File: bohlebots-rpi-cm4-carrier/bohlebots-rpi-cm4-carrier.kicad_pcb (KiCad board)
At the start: 2 copper layers, 32 parts, among them J1 SI-46001-F, J2 power_reference, J3 IO_Conn_02x05, J4 I2C_Conn_1x04, J5 pwr_connector, J6 pwr_connector, K1 Kicker, T1 Taster_LED, T2 Taster_LED, U1 Compute_Module_4_Connectors, U2 USB_Conn_01x05_Pin, U3 DT1446-04SO-7, U5 DT1446-04SO-7, X1 Miromatch

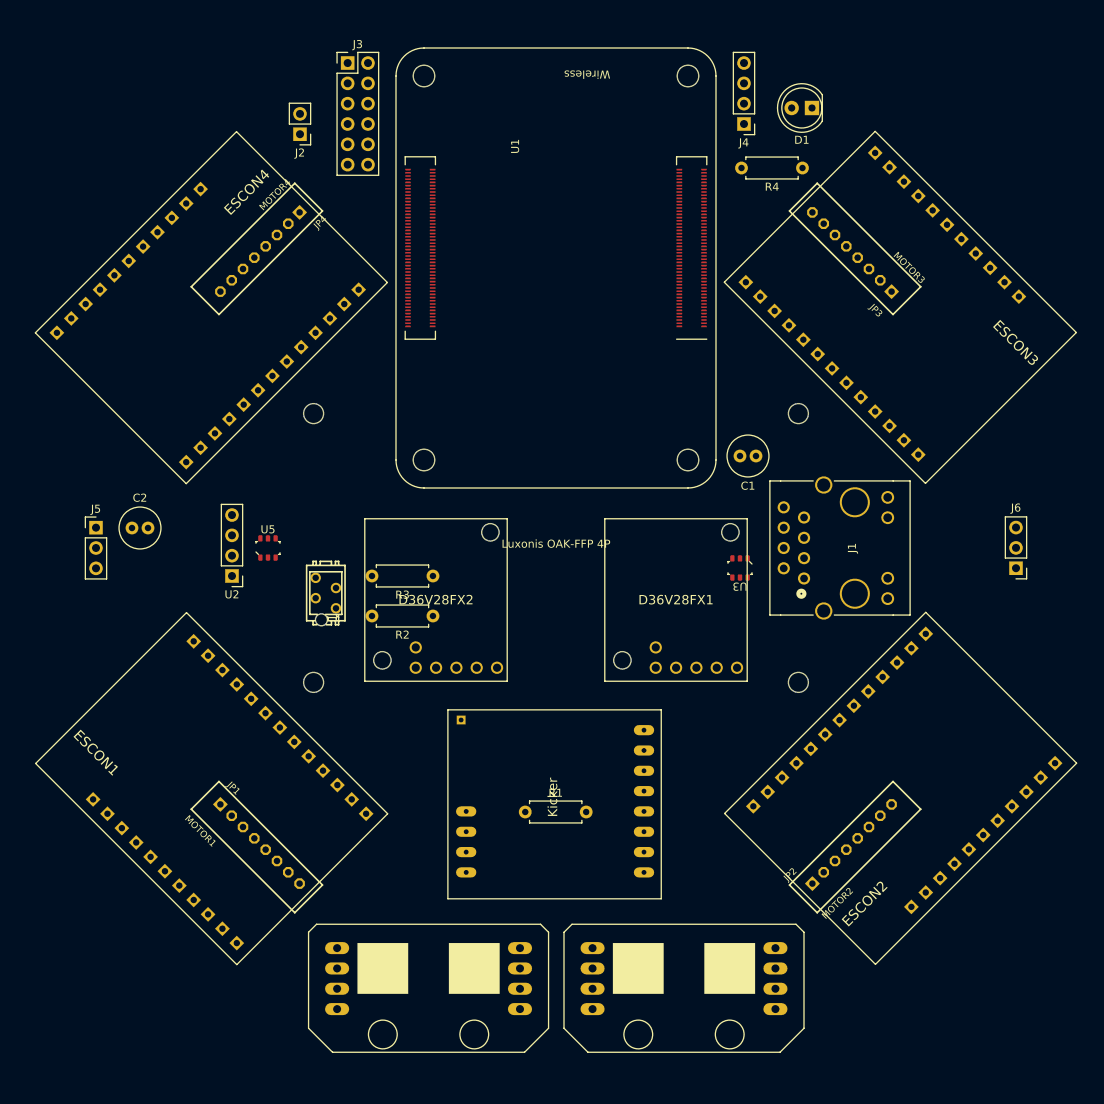
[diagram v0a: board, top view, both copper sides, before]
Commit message: V01 finished.
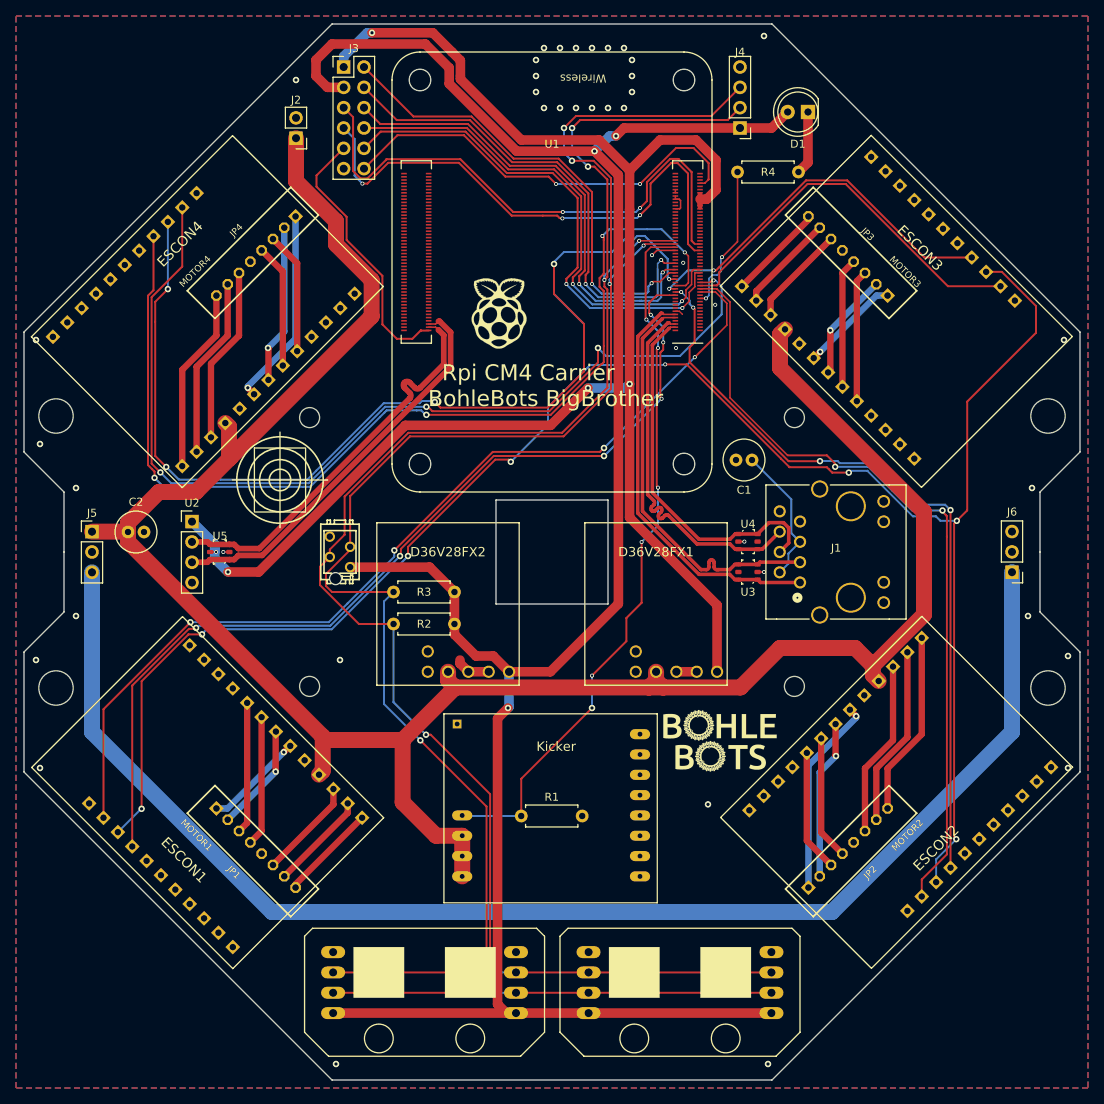
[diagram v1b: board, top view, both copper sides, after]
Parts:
- added G***: LOGO, bohlebots:logo_klein, F.Cu at (126.4, 129.1)
- added G***: LOGO, RPi_Compute_Module_4:logo, F.Cu at (98.9, 75.7)
- added REF**: MountingHole_4.3mm_M4, MountingHole:MountingHole_4.3mm_M4, F.Cu at (167.5, 88.5)
- added REF**: BohlebotsBigBrother_Logo, bohlebots-rpi-cm4-carrier:BohlebotsBigBrother_Logo, F.Cu at (71.5, 96.5)
- added REF**: MountingHole_4.3mm_M4, MountingHole:MountingHole_4.3mm_M4, F.Cu at (43.5, 122.5)
- added REF**: MountingHole_4.3mm_M4, MountingHole:MountingHole_4.3mm_M4, F.Cu at (43.5, 88.5)
- added REFe: MountingHole_4.3mm_M4, MountingHole:MountingHole_4.3mm_M4, F.Cu at (167.5, 122.5)
- added U4: DT1446-04SO-7, bohlebots-rpi-cm4-carrier:SOT26, F.Cu at (130.0, 104.2)
- moved U2 8.44 mm to (60.5, 101.7), turned to 0 degrees
- moved U5 6.05 mm to (64.0, 105.5), turned to 90 degrees
- moved X1 5.44 mm to (77.7, 104.9)
- moved R3 3.35 mm to (93.3, 110.5)
- moved R2 2.87 mm to (93.3, 114.5)
- moved D36V28FX1 2.55 mm to (116.0, 117.9)
- moved D36V28FX2 1.58 mm to (90.0, 117.9)
- moved U3 1.12 mm to (130.0, 108.0), turned to 90 degrees
- moved C1 0.71 mm to (130.5, 94.0)
- moved C2 0.71 mm to (52.5, 103.0)
- moved D1 0.71 mm to (137.5, 50.5)
- moved ESCON1 0.71 mm to (61.5, 136.5)
- moved ESCON2 0.71 mm to (149.5, 136.5)
- moved ESCON3 0.71 mm to (149.5, 74.5)
- moved ESCON4 0.71 mm to (61.5, 74.5)
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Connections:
- ESCON2 pad P15: /DIR1 -> /DIR2
- ESCON2 pad P17: /PWM1 -> /PWM2
- ESCON3 pad P15: /DIR1 -> /DIR3
- ESCON3 pad P17: /PWM1 -> /PWM3
- ESCON4 pad P15: /DIR1 -> /DIR4
- ESCON4 pad P17: /PWM1 -> /PWM4
- T1 pad 1: /3.3v -> 3.3V
- T1 pad 8: /3.3v -> 3.3V
- T2 pad 1: /3.3v -> 3.3V
- T2 pad 8: /3.3v -> 3.3V
- U3 pad 1: /RD_N -> /TD_P
- U3 pad 4: /TD_P -> /TD_N
- U3 pad 6: /RD_P -> /TD_P
- U5 pad 1: /USB_N -> /USB_P
- U5 pad 3: Net-(U5-D2-) -> /USB_N
- U5 pad 4: Net-(U5-D2+) -> /USB_N
- X1 pad 1: /3.3v -> 3.3V
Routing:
- net /ENA: track 0.00 -> 375.8 mm, vias 0 -> 13
- net 3.3V: track 0.00 -> 277.7 mm, vias 0 -> 3
- net 16V: track 0.00 -> 275.4 mm
- net /SCL: track 0.00 -> 239.5 mm, vias 0 -> 6
- net /SDA: track 0.00 -> 237.1 mm, vias 0 -> 6
- net 5V: track 0.00 -> 206.2 mm, vias 0 -> 5
- net Net-(J5-GND): track 0.00 -> 173.6 mm
- net /PWM4: track 0.00 -> 128.2 mm, vias 0 -> 4
- net /DIR4: track 0.00 -> 123.6 mm, vias 0 -> 4
- net /DIR1: track 0.00 -> 118.5 mm, vias 0 -> 4
- net /PWM1: track 0.00 -> 118.1 mm, vias 0 -> 6
- net /DIR2: track 0.00 -> 98.8 mm, vias 0 -> 2
- net /PWM2: track 0.00 -> 95.5 mm, vias 0 -> 4
- net /KICK: track 0.00 -> 89.7 mm, vias 0 -> 6
- net /UART0_TXD: track 0.00 -> 69.5 mm, vias 0 -> 2
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- added copper zone on B.Cu, net GND
- added copper zone on F.Cu, net GND
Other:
- board outline added: 132 x 132 mm
- board text added: "Rpi CM4 Carrier BohleBots BigBrother"
